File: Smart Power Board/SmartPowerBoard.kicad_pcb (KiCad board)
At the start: 13 copper layers, 58.8 x 38 mm, 116 parts, among them J1 430450200, J2 USB_C_Receptacle_USB2.0_16P, J6 430450601, J7 Screw_Terminal_01x04, Q1 FDN338P, Q4 FDN335N, SW1 SW_Push, SW2 SW_Push, SW3 SW_Push, U1 INA3221, U2 TPS561201DDCR, U4 TPS56C230RJER, U5 TPS56C230RJER, U6 RP2040, U7 W25Q32JVSS, U8 TPS561201DDCR, Y1 FL1200138

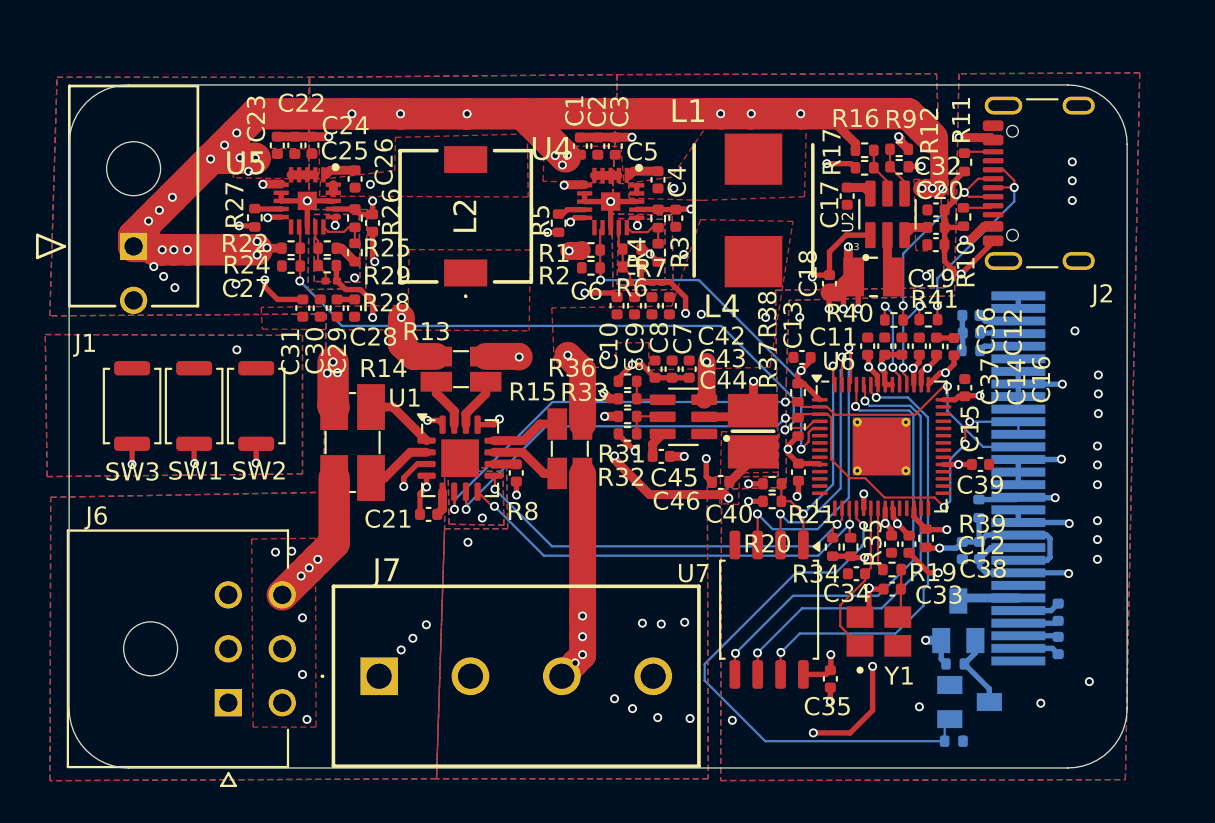
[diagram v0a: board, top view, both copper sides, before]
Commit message: Feat[SmartPowerBoard]: Tapeout
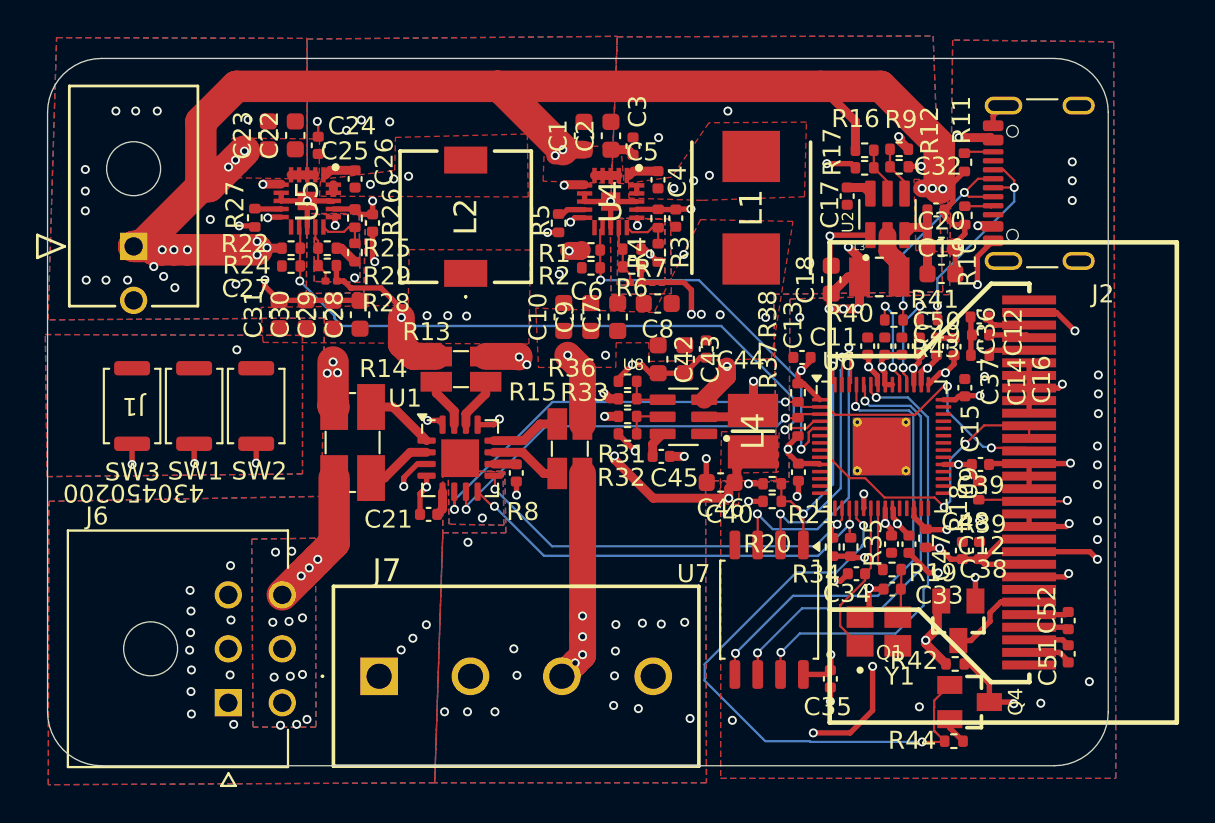
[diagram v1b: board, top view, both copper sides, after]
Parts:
- C1, C10, C18, C19, C2, C20, C22, C23, C28, C29, C30, C31, C42, C43, C46, C7, C8, C9: footprint Capacitor_SMD:C_0402_1005Metric -> Capacitor_SMD:C_0603_1608Metric
- C47, C48, C49, C50, C51, C52, Q1, Q4, R18, R42, R43, R44, U9: moved to F.Cu
- moved C10 3.03 mm to (161.0, 84.2)
- moved C7 2.94 mm to (164.0, 84.2)
- moved C9 2.51 mm to (162.5, 84.2)
- moved C19 1.65 mm to (182.0, 81.8)
- moved C44 1.47 mm to (168.9, 86.0)
- moved C31 1.36 mm to (145.2, 84.1)
- moved C20 1.12 mm to (182.0, 80.3)
- moved U9 1.02 mm to (186.1, 93.4)
- moved R18 1.01 mm to (184.1, 93.9), turned to -90 degrees
- moved C3 0.99 mm to (164.9, 74.7)
- moved C2 0.93 mm to (163.7, 74.2)
- moved C43 0.89 mm to (167.8, 86.6)
- moved C30 0.86 mm to (146.7, 84.1)
- moved C23 0.75 mm to (144.6, 74.1)
- moved C51 0.73 mm to (189.1, 103.0)
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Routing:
- net /12V_{IN}: track 97.3 -> 111.2 mm, vias 34 -> 21
- net Net-(Q1-Pad1): track 4.25 -> 13.5 mm, vias 0 -> 2
- net /OLED Display/RES#: track 79.4 -> 83.2 mm
- net /Inner Buck Converter 4V/4V_{CC}: track 35.6 -> 38.9 mm
- net /MCU/GPIO15: track 31.1 -> 33.2 mm, vias 1 -> 2
- net /OLED Display/V_{BAT}: track 3.40 -> 5.10 mm
- net /Buck Converter 3.3V/3.3V_{OUT}: track 7.92 -> 9.32 mm, vias 2 -> 4
- net /MCU/SDA: track 43.4 -> 42.1 mm, vias 5 -> 4
- net /MCU/3.3V_{CC}: track 146.2 -> 145.0 mm
- net /Buck Converter 5V/5V_{OUT}: track 54.8 -> 55.7 mm, vias 8 -> 9
- net /MCU/SCL: track 38.3 -> 39.0 mm, vias 3 -> 4
- net GND: track 107.6 -> 107.4 mm, vias 64 -> 99
- net /Connectors/3.3V_{OUT}: vias 4 -> 5
- net /Connectors/12V_{OUT}: vias 8 -> 14
- net /Buck Converter 5V/SW: vias 2 -> 4
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- added copper zone on B.Cu, net /Connectors/12V_{OUT}
- added copper zone on In1.Cu, net /Connectors/12V_{OUT}
- added copper zone on In2.Cu, net /Connectors/12V_{OUT}
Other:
- board size 58.8 x 38 mm -> 59 x 39.3 mm
